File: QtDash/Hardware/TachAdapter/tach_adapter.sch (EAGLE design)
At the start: 12 parts, among them IC1 PS2701-1

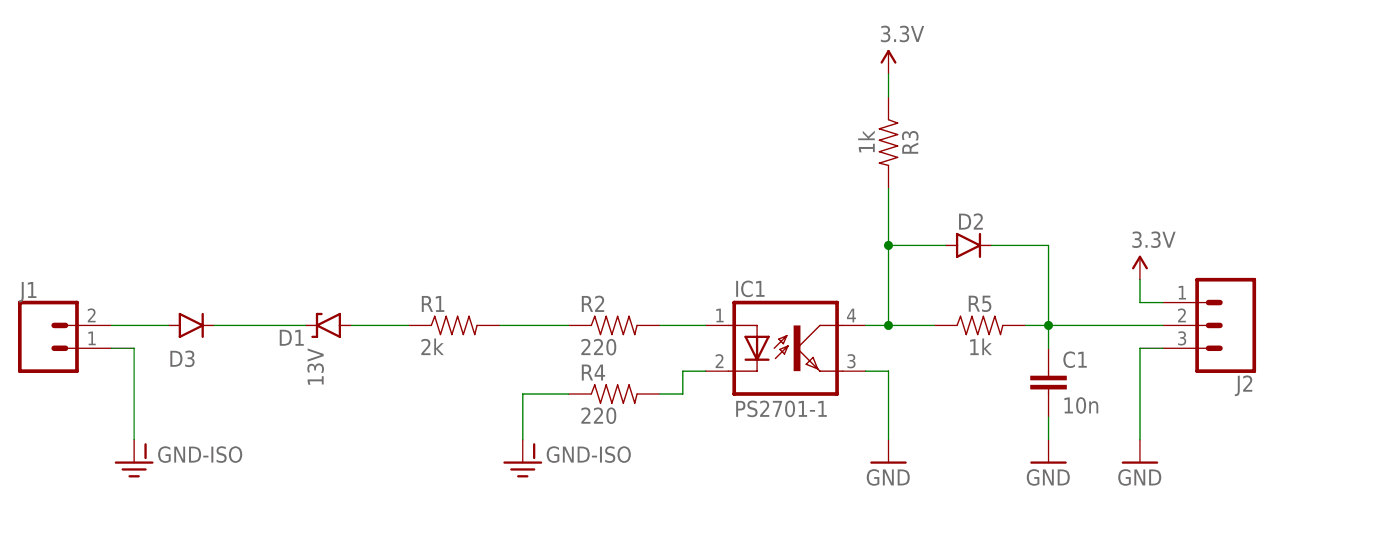
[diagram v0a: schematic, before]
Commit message: bugfix/tach-adapter-updates: 	- updated eagle tach adapter project
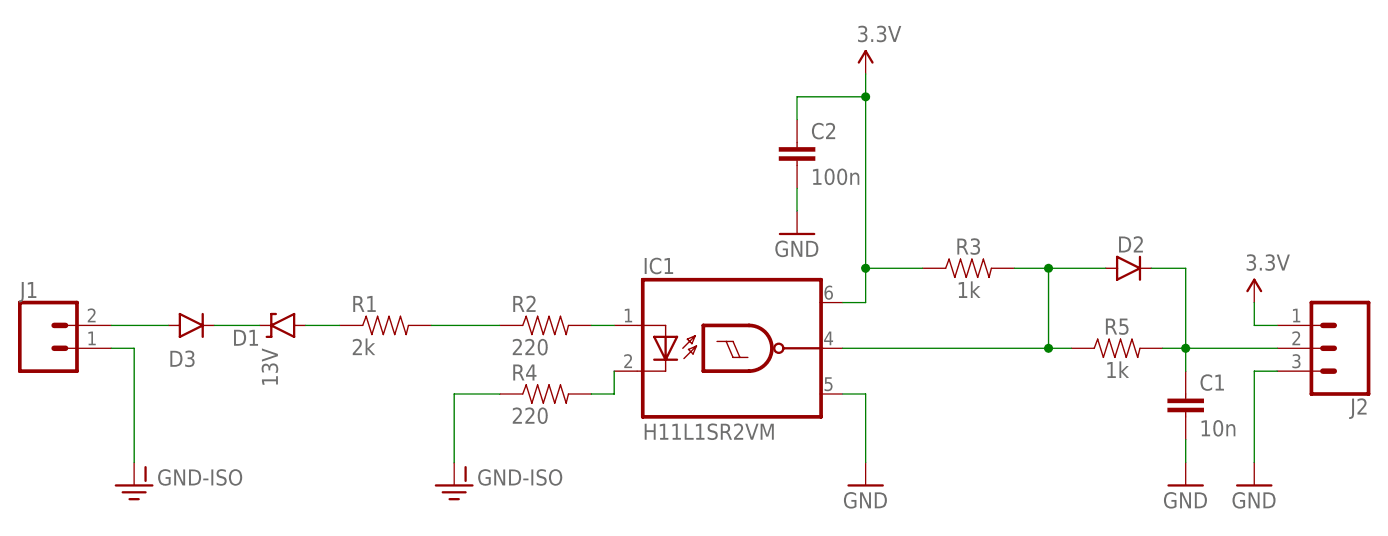
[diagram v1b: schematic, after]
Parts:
- added C2: 100n, digital_dash:CL10B104MB8NNNC
- IC1: value PS2701-1 -> H11L1SR2VM; device tach_adapter:PS2701-1 -> tach_adapter:H11L1SR2VM
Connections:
- net 3.3V: now also C2.1, IC1.VCC
- net GND: now also C2.2, IC1.GND; no longer IC1.EMIT
- net N$7: now also IC1.VOUT; no longer IC1.COL
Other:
- moved on the sheet: C1, D1, D2, J2, R1, R2, R3, R4, R5
